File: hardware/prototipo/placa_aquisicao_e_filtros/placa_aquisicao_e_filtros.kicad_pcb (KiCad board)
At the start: 2 copper layers, 21 parts, among them J1 Conn_01x04, J3 Conn_01x02, J4 Conn_02x04_Counter_Clockwise, U1 Opamp_Quad_Generic, U2 AD620

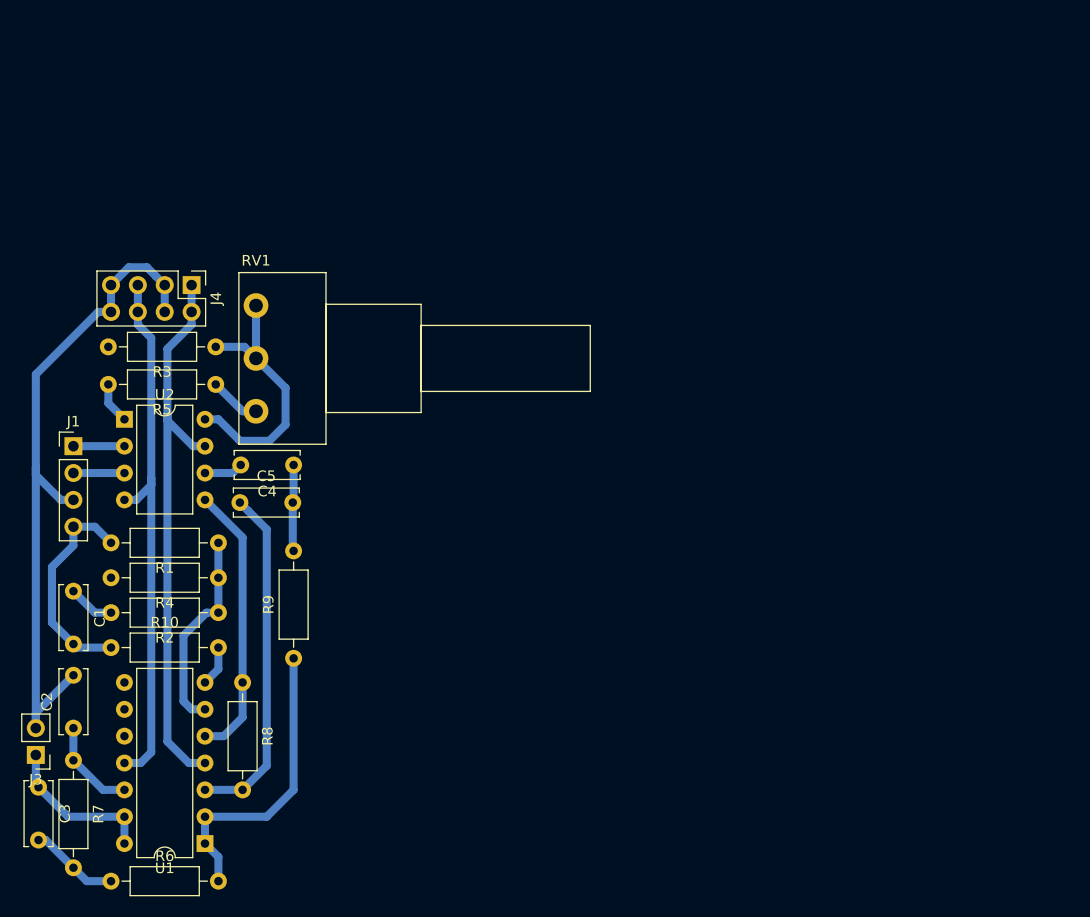
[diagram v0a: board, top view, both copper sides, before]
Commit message: Acquisition prototype board finalized.
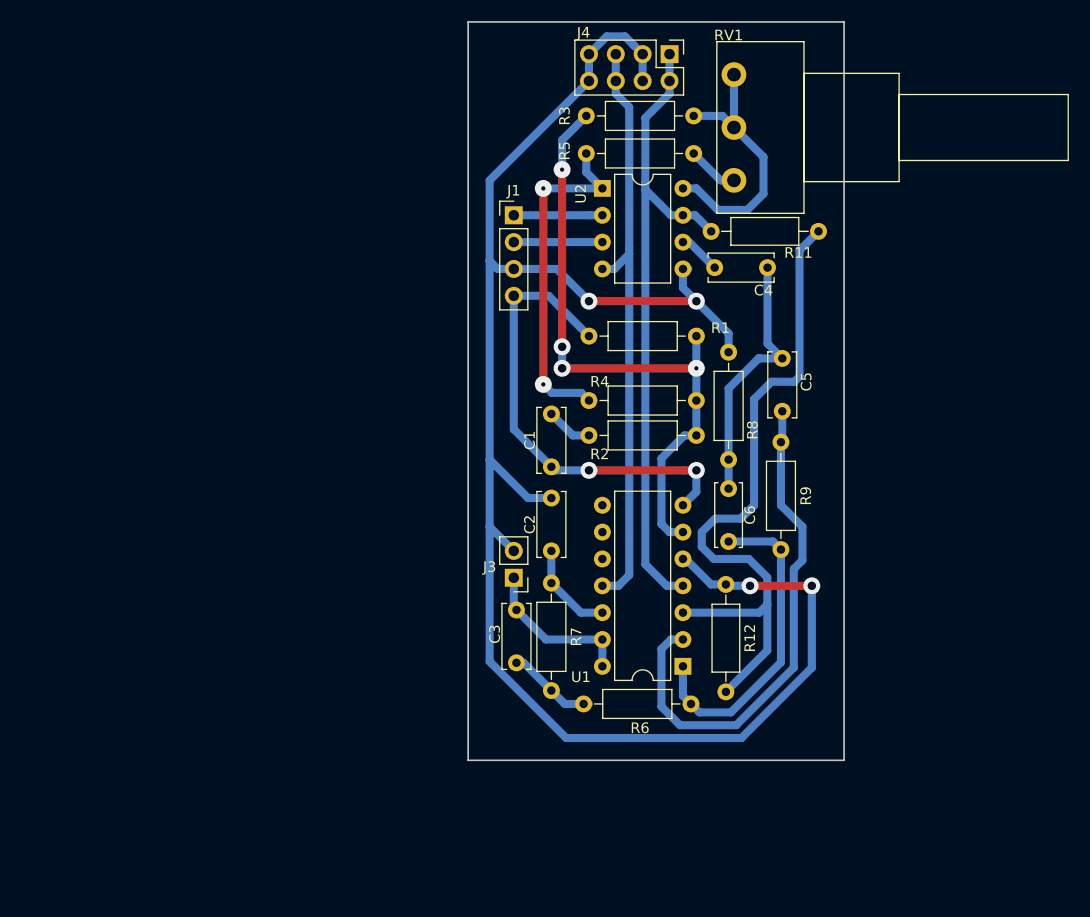
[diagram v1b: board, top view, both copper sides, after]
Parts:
- removed R10: 0R, Resistor_THT:R_Axial_DIN0207_L6.3mm_D2.5mm_P10.16mm_Horizontal
- added C6: 47u, Capacitors_THT:C_Disc_D6.0mm_W2.5mm_P5.00mm, F.Cu at (155.4, 107.8)
- added R11: 130k, Resistors_THT:R_Axial_DIN0207_L6.3mm_D2.5mm_P10.16mm_Horizontal, F.Cu at (153.8, 78.5)
- added R12: 18k, Resistors_THT:R_Axial_DIN0207_L6.3mm_D2.5mm_P10.16mm_Horizontal, F.Cu at (155.2, 122.0)
- R8: value 91k -> 33k
- R9: value 47k -> 150k
- moved R8 55.6 mm to (155.4, 89.9)
- moved C5 52.0 mm to (160.5, 95.5), turned to 90 degrees
- moved R9 50.4 mm to (160.4, 98.4), turned to 270 degrees
- moved J4 50.2 mm to (149.9, 61.7)
- moved R3 50.2 mm to (152.1, 67.6)
- moved RV1 50.2 mm to (156.0, 73.7)
- moved U2 50.2 mm to (143.5, 74.4)
- moved R5 50.2 mm to (152.1, 71.1)
- moved R1 49.3 mm to (152.4, 88.4)
- moved C4 48.6 mm to (159.1, 81.9)
- moved C1 48.2 mm to (138.7, 95.8)
- moved C2 48.2 mm to (138.7, 108.7)
- moved C3 48.2 mm to (135.4, 114.3)
- moved R2 48.2 mm to (152.4, 97.8)
- moved R4 48.2 mm to (152.4, 94.5)
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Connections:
- J1 pad 1: right_electrode -> left_electrode
- J1 pad 2: left_electrode -> right_electrode
- R8 pad 2: Net-(C5-Pad1) -> Net-(C4-Pad1)
- R9 pad 1: out2 -> Net-(C5-Pad1)
- R9 pad 2: Net-(C4-Pad1) -> out2
- U1 pad 2: out2 -> Net-(C5-Pad1)
- U1 pad 3: Net-(C5-Pad1) -> Net-(R11-Pad2)
- U1 pad 7: Net-(R10-Pad2) -> ref_electrode
- U2 pad 2: right_electrode -> left_electrode
- U2 pad 3: left_electrode -> right_electrode
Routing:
- net GNDA: track 92.6 -> 169.4 mm, vias 0 -> 4
- net Net-(R11-Pad2): track 0.00 -> 65.2 mm
- net Net-(R1-Pad1): track 19.4 -> 60.8 mm, vias 0 -> 4
- net Net-(R4-Pad2): track 3.93 -> 33.0 mm, vias 0 -> 2
- net ref_electrode: track 20.7 -> 44.0 mm, vias 0 -> 2
- net Net-(C4-Pad1): track 8.19 -> 25.0 mm
- net Net-(C5-Pad1): track 32.7 -> 48.8 mm
- net +9V: track 53.7 -> 61.5 mm
- net -9V: track 51.4 -> 55.9 mm
- net Net-(R10-Pad2): track 3.83 -> 0.00 mm
- net right_electrode: track 4.83 -> 8.38 mm
- net left_electrode: track 4.83 -> 8.38 mm
- net out2: track 28.5 -> 30.6 mm
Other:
- board outline added: 35.6 x 69.8 mm
